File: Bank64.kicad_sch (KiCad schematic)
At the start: 2 parts, among them U1 XCKU5P-FFVB676

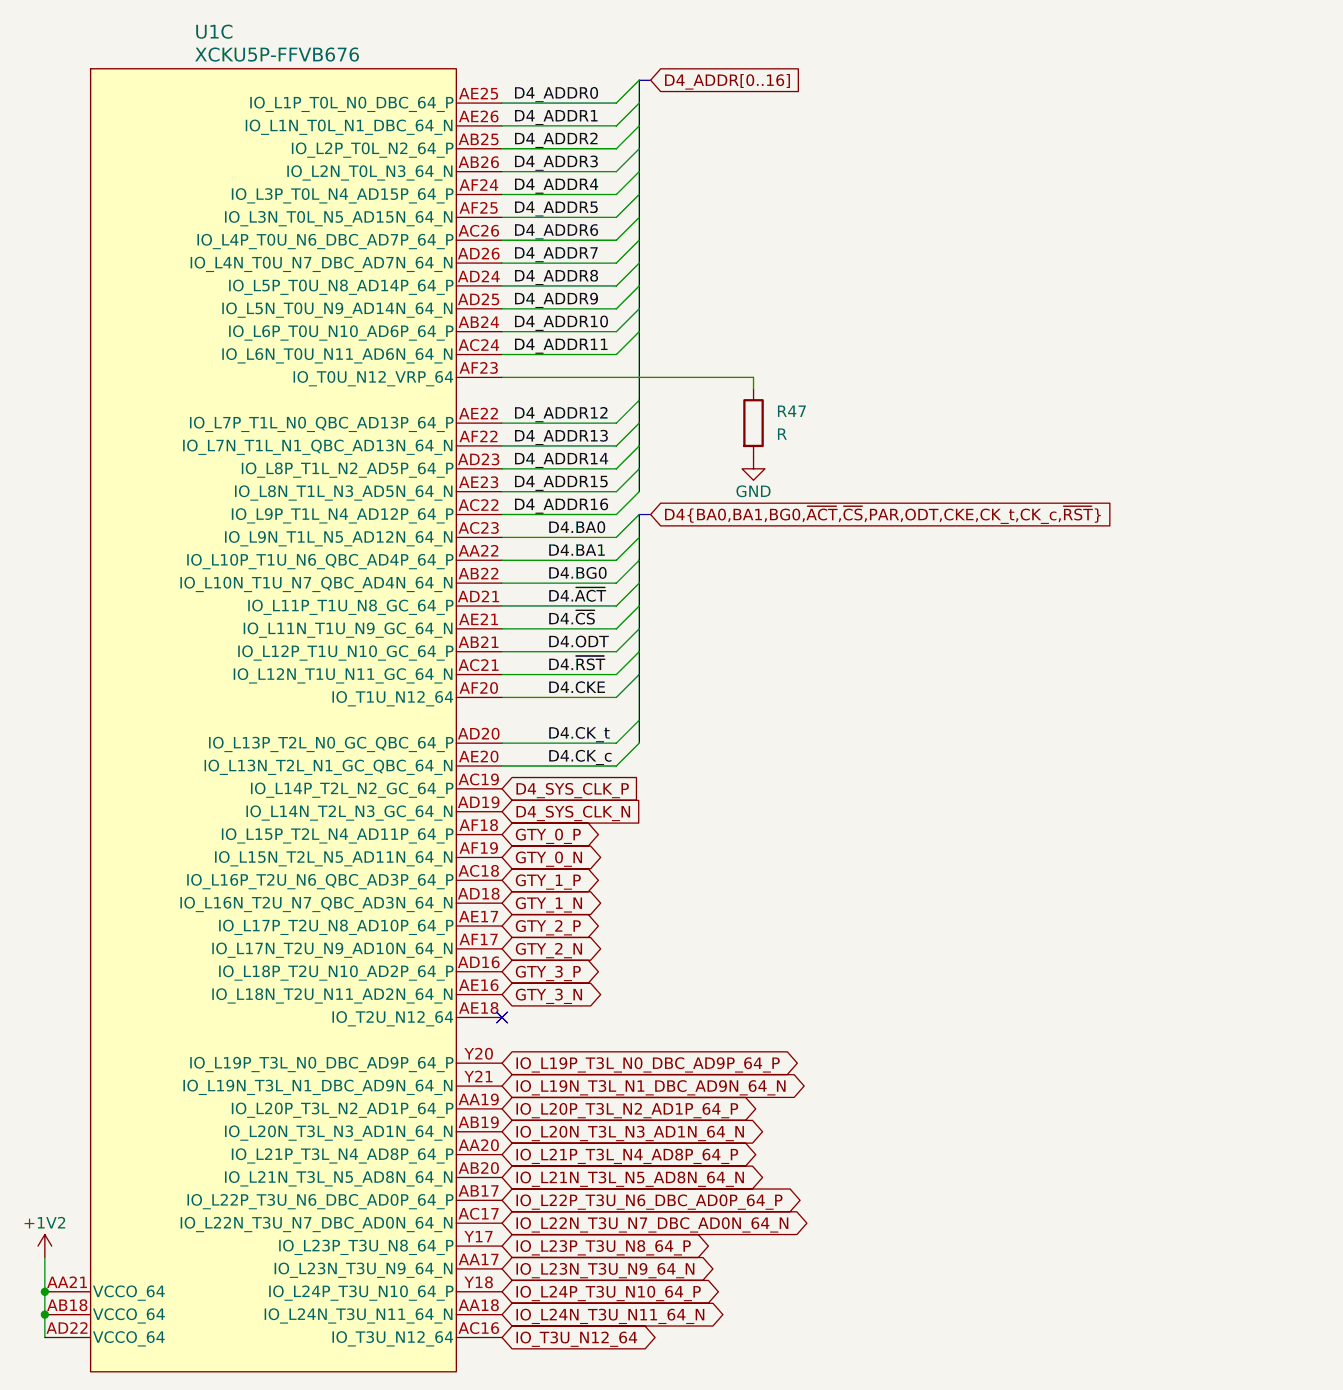
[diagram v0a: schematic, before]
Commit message: pushing the schematics works
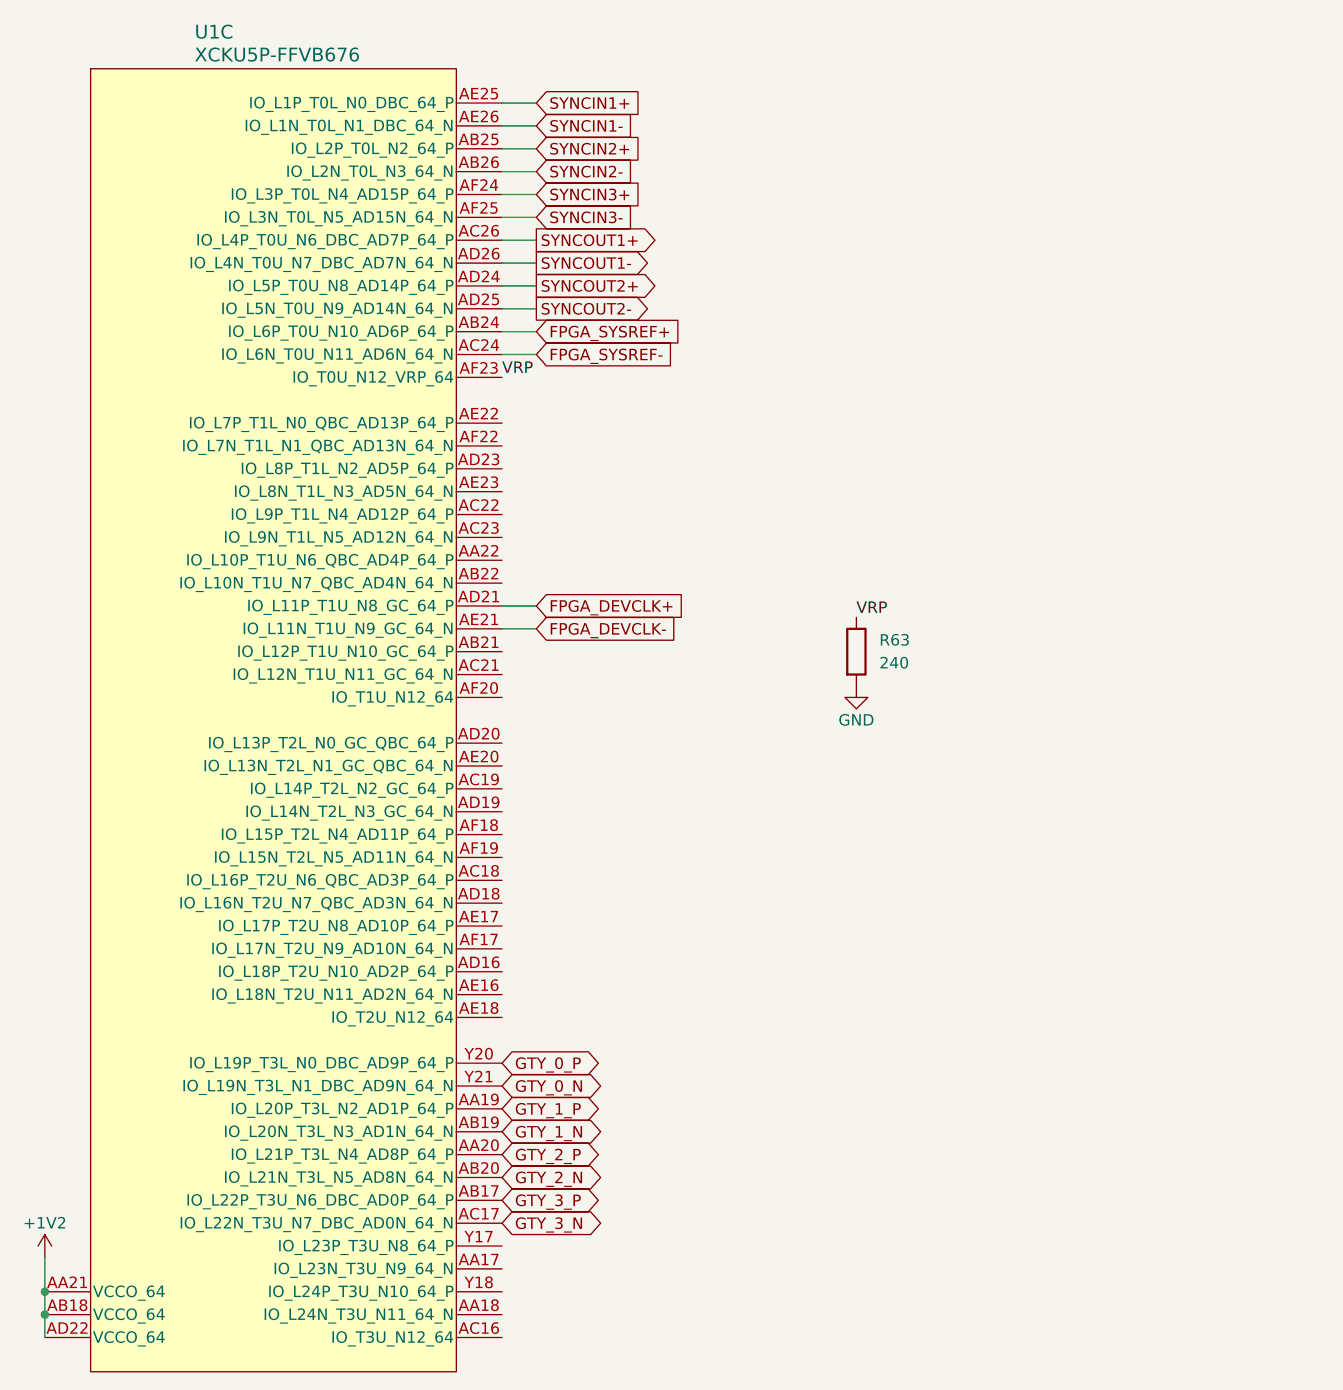
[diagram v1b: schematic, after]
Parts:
- removed R47: R, Resistor_SMD:R_0201_0603Metric, symbol Device:R
- added R63: 240, Resistor_SMD:R_0201_0603Metric, symbol Device:R
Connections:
- net IO_L19N_T3L_N1_DBC_AD9N_64_N is gone; now on net GTY_0_N: U1.Y21 (IO_L19N_T3L_N1_DBC_AD9N_64_N)
- net IO_L19P_T3L_N0_DBC_AD9P_64_P is gone; now on net GTY_0_P: U1.Y20 (IO_L19P_T3L_N0_DBC_AD9P_64_P)
- net IO_L20N_T3L_N3_AD1N_64_N is gone; now on net GTY_1_N: U1.AB19 (IO_L20N_T3L_N3_AD1N_64_N)
- net IO_L20P_T3L_N2_AD1P_64_P is gone; now on net GTY_1_P: U1.AA19 (IO_L20P_T3L_N2_AD1P_64_P)
- net IO_L21N_T3L_N5_AD8N_64_N is gone; now on net GTY_2_N: U1.AB20 (IO_L21N_T3L_N5_AD8N_64_N)
- net IO_L21P_T3L_N4_AD8P_64_P is gone; now on net GTY_2_P: U1.AA20 (IO_L21P_T3L_N4_AD8P_64_P)
- net IO_L22N_T3U_N7_DBC_AD0N_64_N is gone; now on net GTY_3_N: U1.AC17 (IO_L22N_T3U_N7_DBC_AD0N_64_N)
- net IO_L22P_T3U_N6_DBC_AD0P_64_P is gone; now on net GTY_3_P: U1.AB17 (IO_L22P_T3U_N6_DBC_AD0P_64_P)
- net GND: now also R63.2
- net GTY_0_N: no longer U1.AF19 (IO_L15N_T2L_N5_AD11N_64_N)
- net GTY_0_P: no longer U1.AF18 (IO_L15P_T2L_N4_AD11P_64_P)
- net GTY_1_N: no longer U1.AD18 (IO_L16N_T2U_N7_QBC_AD3N_64_N)
- net GTY_1_P: no longer U1.AC18 (IO_L16P_T2U_N6_QBC_AD3P_64_P)
- net GTY_2_N: no longer U1.AF17 (IO_L17N_T2U_N9_AD10N_64_N)
- net GTY_2_P: no longer U1.AE17 (IO_L17P_T2U_N8_AD10P_64_P)
- net GTY_3_N: no longer U1.AE16 (IO_L18N_T2U_N11_AD2N_64_N)
- net GTY_3_P: no longer U1.AD16 (IO_L18P_T2U_N10_AD2P_64_P)
- net VRP: now reaches U1.AF23 (IO_T0U_N12_VRP_64)
- net VRP: now also R63.1
- net D4.BA0: no longer names the net of U1.AC23 (IO_L9N_T1L_N5_AD12N_64_N)
- net D4.BA1: no longer names the net of U1.AA22 (IO_L10P_T1U_N6_QBC_AD4P_64_P)
- net D4.BG0: no longer names the net of U1.AB22 (IO_L10N_T1U_N7_QBC_AD4N_64_N)
- net D4.CKE: no longer names the net of U1.AF20 (IO_T1U_N12_64)
- net D4.CK_c: no longer names the net of U1.AE20 (IO_L13N_T2L_N1_GC_QBC_64_N)
- net D4.CK_t: no longer names the net of U1.AD20 (IO_L13P_T2L_N0_GC_QBC_64_P)
- net D4.ODT: no longer names the net of U1.AB21 (IO_L12P_T1U_N10_GC_64_P)
- net D4.~{ACT} renamed FPGA_DEVCLK+
- net D4.~{CS} renamed FPGA_DEVCLK-
- net D4.~{RST}: no longer names the net of U1.AC21 (IO_L12N_T1U_N11_GC_64_N)
- net D4_ADDR0 renamed SYNCIN1+
- net D4_ADDR1 renamed SYNCIN1-
- net D4_ADDR10 renamed FPGA_SYSREF+
- net D4_ADDR11 renamed FPGA_SYSREF-
- net D4_ADDR12: no longer names the net of U1.AE22 (IO_L7P_T1L_N0_QBC_AD13P_64_P)
- net D4_ADDR13: no longer names the net of U1.AF22 (IO_L7N_T1L_N1_QBC_AD13N_64_N)
- net D4_ADDR14: no longer names the net of U1.AD23 (IO_L8P_T1L_N2_AD5P_64_P)
- net D4_ADDR15: no longer names the net of U1.AE23 (IO_L8N_T1L_N3_AD5N_64_N)
- net D4_ADDR16: no longer names the net of U1.AC22 (IO_L9P_T1L_N4_AD12P_64_P)
- net D4_ADDR2 renamed SYNCIN2+
- net D4_ADDR3 renamed SYNCIN2-
- net D4_ADDR4 renamed SYNCIN3+
- net D4_ADDR5 renamed SYNCIN3-
- net D4_ADDR6 renamed SYNCOUT1+
- net D4_ADDR7 renamed SYNCOUT1-
- net D4_ADDR8 renamed SYNCOUT2+
- net D4_ADDR9 renamed SYNCOUT2-
- net D4_SYS_CLK_N: no longer names the net of U1.AD19 (IO_L14N_T2L_N3_GC_64_N)
- net D4_SYS_CLK_P: no longer names the net of U1.AC19 (IO_L14P_T2L_N2_GC_64_P)
- net IO_L23N_T3U_N9_64_N: no longer names the net of U1.AA17 (IO_L23N_T3U_N9_64_N)
- net IO_L23P_T3U_N8_64_P: no longer names the net of U1.Y17 (IO_L23P_T3U_N8_64_P)
- net IO_L24N_T3U_N11_64_N: no longer names the net of U1.AA18 (IO_L24N_T3U_N11_64_N)
- net IO_L24P_T3U_N10_64_P: no longer names the net of U1.Y18 (IO_L24P_T3U_N10_64_P)
- net IO_T3U_N12_64: no longer names the net of U1.AC16 (IO_T3U_N12_64)
- no-connect marks 1 -> 0
